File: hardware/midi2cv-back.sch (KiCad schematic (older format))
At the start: 3 parts

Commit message: Add amplifier circuits for DACs
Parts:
- removed U?: STM32F103C8Tx, Package_QFP:LQFP-48_7x7mm_P0.5mm, symbol MCU_ST_STM32F1:STM32F103C8Tx
- added U?: STM32F410RBTx, Package_QFP:LQFP-64_10x10mm_P0.5mm, symbol MCU_ST_STM32F4:STM32F410RBTx
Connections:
- wire segments 29 -> 33
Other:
- moved on the sheet: C?, U?
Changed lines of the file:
@@
 L power:GND #PWR?
 U 1 1 60A4D09B
-P 4250 4750
-F 0 "#PWR?" H 4250 4500 50  0001 C CNN
-F 1 "GND" H 4255 4577 50  0000 C CNN
-F 2 "" H 4250 4750 50  0001 C CNN
-F 3 "" H 4250 4750 50  0001 C CNN
-	1    4250 4750
+P 2350 4850
+F 0 "#PWR?" H 2350 4600 50  0001 C CNN
+F 1 "GND" H 2355 4677 50  0000 C CNN
+F 2 "" H 2350 4850 50  0001 C CNN
+F 3 "" H 2350 4850 50  0001 C CNN
+	1    2350 4850
 	1    0    0    -1
 $EndComp
 Wire Wire Line
-	3850 4100 3850 4200
+	1950 4200 1950 4300
 Wire Wire Line
-	3850 4600 4250 4600
+	1950 4700 2350 4700
 Wire Wire Line
-	4250 4600 4250 4500
-Connection ~ 3850 4200
+	2350 4700 2350 4600
+Connection ~ 1950 4300
 Wire Wire Line
-	3850 4200 3850 4300
-Connection ~ 3850 4300
+	1950 4300 1950 4400
+Connection ~ 1950 4400
 Wire Wire Line
-	3850 4300 3850 4600
+	1950 4400 1950 4700
 Wire Wire Line
-	4250 4600 4250 4750
-Connection ~ 4250 4600
+	2350 4700 2350 4850
+Connection ~ 2350 4700
 Wire Wire Line
-	4250 4600 4650 4600
+	2350 4700 2750 4700
 Wire Wire Line
-	4650 4600 4650 4300
+	2750 4700 2750 4400
 $Comp
 L power:+3.3V #PWR?
 U 1 1 60A52E41
-P 4250 3900
-F 0 "#PWR?" H 4250 3750 50  0001 C CNN
-F 1 "+3.3V" H 4265 4073 50  0000 C CNN
-F 2 "" H 4250 3900 50  0001 C CNN
-F 3 "" H 4250 3900 50  0001 C CNN
-	1    4250 3900
+P 2350 4000
+F 0 "#PWR?" H 2350 3850 50  0001 C CNN
+F 1 "+3.3V" H 2365 4173 50  0000 C CNN
+F 2 "" H 2350 4000 50  0001 C CNN
+F 3 "" H 2350 4000 50  0001 C CNN
+	1    2350 4000
 	1    0    0    -1
 $EndComp
 Wire Wire Line
-	4650 4100 5300 4100
+	2750 4200 3400 4200
 Wire Wire Line
-	4650 4200 5300 4200
+	2750 4300 3400 4300
 $Comp
 L power:+3.3V #PWR?
 U 1 1 60A58EE0
-P 3350 3950
-F 0 "#PWR?" H 3350 3800 50  0001 C CNN
-F 1 "+3.3V" H 3365 4123 50  0000 C CNN
-F 2 "" H 3350 3950 50  0001 C CNN
-F 3 "" H 3350 3950 50  0001 C CNN
-	1    3350 3950
+P 1450 4050
+F 0 "#PWR?" H 1450 3900 50  0001 C CNN
+F 1 "+3.3V" H 1465 4223 50  0000 C CNN
+F 2 "" H 1450 4050 50  0001 C CNN
+F 3 "" H 1450 4050 50  0001 C CNN
+	1    1450 4050
 	1    0    0    -1
 $EndComp
@@
 L power:GND #PWR?
 U 1 1 60A592F0
-P 3350 4250
-F 0 "#PWR?" H 3350 4000 50  0001 C CNN
-F 1 "GND" H 3355 4077 50  0000 C CNN
-F 2 "" H 3350 4250 50  0001 C CNN
-F 3 "" H 3350 4250 50  0001 C CNN
-	1    3350 4250
+P 1450 4350
+F 0 "#PWR?" H 1450 4100 50  0001 C CNN
+F 1 "GND" H 1455 4177 50  0000 C CNN
+F 2 "" H 1450 4350 50  0001 C CNN
+F 3 "" H 1450 4350 50  0001 C CNN
+	1    1450 4350
 	1    0    0    -1
 $EndComp
@@
 L Device:C C?
 U 1 1 60A598C4
-P 3350 4100
-F 0 "C?" H 3465 4146 50  0000 L CNN
-F 1 "100n" H 3465 4055 50  0000 L CNN
-F 2 "" H 3388 3950 50  0001 C CNN
-F 3 "~" H 3350 4100 50  0001 C CNN
-	1    3350 4100
+P 1450 4200
+F 0 "C?" H 1565 4246 50  0000 L CNN
+F 1 "100n" H 1565 4155 50  0000 L CNN
+F 2 "" H 1488 4050 50  0001 C CNN
+F 3 "~" H 1450 4200 50  0001 C CNN
+	1    1450 4200
 	1    0    0    -1
 $EndComp
@@
 L power:+3.3V #PWR?
 U 1 1 60A5CF6A
-P 6000 1800
-F 0 "#PWR?" H 6000 1650 50  0001 C CNN
-F 1 "+3.3V" H 6015 1973 50  0000 C CNN
-F 2 "" H 6000 1800 50  0001 C CNN
-F 3 "" H 6000 1800 50  0001 C CNN
-	1    6000 1800
+P 5600 1400
+F 0 "#PWR?" H 5600 1250 50  0001 C CNN
+F 1 "+3.3V" H 5615 1573 50  0000 C CNN
+F 2 "" H 5600 1400 50  0001 C CNN
+F 3 "" H 5600 1400 50  0001 C CNN
+	1    5600 1400
 	1    0    0    -1
 $EndComp
 Wire Wire Line
-	6000 1800 6000 1900
+	5350 1700 5350 1500
 Wire Wire Line
-	5800 2100 5800 1900
+	5350 1500 5450 1500
+Connection ~ 5550 1500
 Wire Wire Line
-	5800 1900 5900 1900
-Connection ~ 6000 1900
+	5550 1500 5550 1700
 Wire Wire Line
-	6000 1900 6000 2100
+	5450 1700 5450 1500
+Connection ~ 5450 1500
 Wire Wire Line
-	5900 2100 5900 1900
-Connection ~ 5900 1900
+	5450 1500 5550 1500
 Wire Wire Line
-	5900 1900 6000 1900
+	5650 1700 5650 1500
 Wire Wire Line
-	6100 2100 6100 1900
+	5650 1500 5600 1500
 Wire Wire Line
-	6100 1900 6000 1900
+	5750 1700 5750 1500
 Wire Wire Line
-	6200 2100 6200 1900
+	5750 1500 5650 1500
+Connection ~ 5650 1500
 Wire Wire Line
-	6200 1900 6100 1900
-Connection ~ 6100 1900
-Wire Wire Line
-	5900 5100 5900 5300
+	5450 5300 5450 5500
 $Comp
 L Memory_EEPROM:CAT24C256 U?
 U 1 1 60A44E16
-P 4250 4200
-F 0 "U?" H 3850 4600 50  0000 C CNN
-F 1 "AT24C256C" H 3850 4500 50  0000 C CNN
-F 2 "" H 4250 4200 50  0001 C CNN
-F 3 "https://www.onsemi.cn/PowerSolutions/document/CAT24C256-D.PDF" H 4250 4200 50  0001 C CNN
-	1    4250 4200
+P 2350 4300
+F 0 "U?" H 1950 4700 50  0000 C CNN
+F 1 "AT24C256C" H 1950 4600 50  0000 C CNN
+F 2 "" H 2350 4300 50  0001 C CNN
+F 3 "https://www.onsemi.cn/PowerSolutions/document/CAT24C256-D.PDF" H 2350 4300 50  0001 C CNN
+	1    2350 4300
 	1    0    0    -1
 $EndComp
 Wire Wire Line
-	5800 5100 5800 5300
+	5350 5300 5350 5500
 Wire Wire Line
-	5800 5300 5900 5300
+	5350 5500 5450 5500
 Wire Wire Line
-	6000 5300 6000 5100
-Connection ~ 5900 5300
+	5550 5500 5550 5300
+Connection ~ 5450 5500
 Wire Wire Line
-	6000 5300 6100 5300
+	5550 5500 5650 5500
 Wire Wire Line
-	6100 5300 6100 5100
-Connection ~ 6000 5300
-$Comp
-L MCU_ST_STM32F1:STM32F103C8Tx U?
-U 1 1 60A44151
-P 6000 3600
-F 0 "U?" H 6550 2050 50  0000 C CNN
-F 1 "STM32F103C8Tx" H 6550 1950 50  0000 C CNN
-F 2 "Package_QFP:LQFP-48_7x7mm_P0.5mm" H 5400 2200 50  0001 R CNN
-F 3 "http://www.st.com/st-web-ui/static/active/en/resource/technical/document/datasheet/CD00161566.pdf" H 6000 3600 50  0001 C CNN
-	1    6000 3600
-	1    0    0    -1
-$EndComp
+	5650 5500 5650 5300
+Connection ~ 5550 5500
 $Comp
 L power:GND #PWR?
 U 1 1 60A664FC
-P 5950 5400
-F 0 "#PWR?" H 5950 5150 50  0001 C CNN
-F 1 "GND" H 5955 5227 50  0000 C CNN
-F 2 "" H 5950 5400 50  0001 C CNN
-F 3 "" H 5950 5400 50  0001 C CNN
-	1    5950 5400
+P 5550 5600
+F 0 "#PWR?" H 5550 5350 50  0001 C CNN
+F 1 "GND" H 5555 5427 50  0000 C CNN
+F 2 "" H 5550 5600 50  0001 C CNN
+F 3 "" H 5550 5600 50  0001 C CNN
+	1    5550 5600
 	1    0    0    -1
 $EndComp
-Wire Wire Line
-	5900 5300 5950 5300
-Wire Wire Line
-	5950 5300 5950 5400
-Connection ~ 5950 5300
-Wire Wire Line
-	5950 5300 6000 5300
-Text GLabel 6600 3900 2    50   Input ~ 0
+Text GLabel 3500 5700 2    50   Input ~ 0
 spi1_sck
 Text GLabel 8500 2600 0    50   Input ~ 0
 spi1_sck
-Text GLabel 6600 3800 2    50   Input ~ 0
+Text GLabel 3500 5600 2    50   Input ~ 0
 spi1_nss
 Text GLabel 8500 2750 0    50   Input ~ 0
 spi1_nss
-Text GLabel 6600 4100 2    50   Input ~ 0
+Text GLabel 3500 5900 2    50   Input ~ 0
 spi1_mosi
 Text GLabel 8500 2450 0    50   Input ~ 0
 spi1_mosi
-Text GLabel 5300 4400 0    50   Input ~ 0
+Text GLabel 3900 5050 0    50   Input ~ 0
 i2c2_scl
-Text GLabel 5300 4500 0    50   Input ~ 0
+Text GLabel 3900 5150 0    50   Input ~ 0
 i2c2_sda
 Text GLabel 8500 4250 0    50   Input ~ 0
@@
 Text GLabel 8500 4450 0    50   Input ~ 0
 i2c2_sda
+$Comp
+L MCU_ST_STM32F4:STM32F410RBTx U?
+U 1 1 60B028B6
+P 5550 3500
+F 0 "U?" H 6150 1650 50  0000 C CNN
+F 1 "STM32F410RBTx" H 6150 1550 50  0000 C CNN
+F 2 "Package_QFP:LQFP-64_10x10mm_P0.5mm" H 4950 1800 50  0001 R CNN
+F 3 "http://www.st.com/st-web-ui/static/active/en/resource/technical/document/datasheet/DM00214043.pdf" H 5550 3500 50  0001 C CNN
+	1    5550 3500
+	1    0    0    -1
+$EndComp
+Wire Wire Line
+	5750 1500 5850 1500
+Wire Wire Line
+	5850 1500 5850 1700
+Connection ~ 5750 1500
+Wire Wire Line
+	5600 1500 5600 1400
+Connection ~ 5600 1500
+Wire Wire Line
+	5600 1500 5550 1500
+Wire Wire Line
+	5650 5500 5750 5500
+Wire Wire Line
+	5750 5500 5750 5300
+Connection ~ 5650 5500
+Wire Wire Line
+	5450 5500 5550 5500
+Wire Wire Line
+	5550 5500 5550 5600
 $EndSCHEMATC

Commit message: Move to single schema tree
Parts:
- removed U?: STM32F410RBTx, Package_QFP:LQFP-64_10x10mm_P0.5mm, symbol MCU_ST_STM32F4:STM32F410RBTx
- added U?: STM32F401RBTx, Package_QFP:LQFP-64_10x10mm_P0.5mm, symbol MCU_ST_STM32F4:STM32F401RBTx
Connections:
- wire segments 33 -> 30
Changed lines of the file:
@@
 $Descr A4 11693 8268
 encoding utf-8
-Sheet 1 3
+Sheet 2 5
 Title ""
 Date ""
@@
 L power:+3.3V #PWR?
 U 1 1 60A5CF6A
-P 5600 1400
-F 0 "#PWR?" H 5600 1250 50  0001 C CNN
-F 1 "+3.3V" H 5615 1573 50  0000 C CNN
-F 2 "" H 5600 1400 50  0001 C CNN
-F 3 "" H 5600 1400 50  0001 C CNN
-	1    5600 1400
-	1    0    0    -1
-$EndComp
-Wire Wire Line
-	5350 1700 5350 1500
-Wire Wire Line
-	5350 1500 5450 1500
-Connection ~ 5550 1500
-Wire Wire Line
-	5550 1500 5550 1700
-Wire Wire Line
-	5450 1700 5450 1500
-Connection ~ 5450 1500
-Wire Wire Line
-	5450 1500 5550 1500
-Wire Wire Line
-	5650 1700 5650 1500
-Wire Wire Line
-	5650 1500 5600 1500
-Wire Wire Line
-	5750 1700 5750 1500
-Wire Wire Line
-	5750 1500 5650 1500
-Connection ~ 5650 1500
+P 5550 1600
+F 0 "#PWR?" H 5550 1450 50  0001 C CNN
+F 1 "+3.3V" H 5565 1773 50  0000 C CNN
+F 2 "" H 5550 1600 50  0001 C CNN
+F 3 "" H 5550 1600 50  0001 C CNN
+	1    5550 1600
+	1    0    0    -1
+$EndComp
 Wire Wire Line
 	5450 5300 5450 5500
@@
 	1    0    0    -1
 $EndComp
-Text GLabel 3500 5700 2    50   Input ~ 0
+Text GLabel 3700 3650 2    50   Input ~ 0
 spi1_sck
 Text GLabel 8500 2600 0    50   Input ~ 0
 spi1_sck
-Text GLabel 3500 5600 2    50   Input ~ 0
+Text GLabel 3700 3550 2    50   Input ~ 0
 spi1_nss
 Text GLabel 8500 2750 0    50   Input ~ 0
 spi1_nss
-Text GLabel 3500 5900 2    50   Input ~ 0
+Text GLabel 3700 3850 2    50   Input ~ 0
 spi1_mosi
 Text GLabel 8500 2450 0    50   Input ~ 0
 spi1_mosi
-Text GLabel 3900 5050 0    50   Input ~ 0
+Text GLabel 4100 3000 0    50   Input ~ 0
 i2c2_scl
-Text GLabel 3900 5150 0    50   Input ~ 0
+Text GLabel 4100 3100 0    50   Input ~ 0
 i2c2_sda
 Text GLabel 8500 4250 0    50   Input ~ 0
@@
 Text GLabel 8500 4450 0    50   Input ~ 0
 i2c2_sda
-$Comp
-L MCU_ST_STM32F4:STM32F410RBTx U?
-U 1 1 60B028B6
-P 5550 3500
-F 0 "U?" H 6150 1650 50  0000 C CNN
-F 1 "STM32F410RBTx" H 6150 1550 50  0000 C CNN
-F 2 "Package_QFP:LQFP-64_10x10mm_P0.5mm" H 4950 1800 50  0001 R CNN
-F 3 "http://www.st.com/st-web-ui/static/active/en/resource/technical/document/datasheet/DM00214043.pdf" H 5550 3500 50  0001 C CNN
-	1    5550 3500
-	1    0    0    -1
-$EndComp
-Wire Wire Line
-	5750 1500 5850 1500
-Wire Wire Line
-	5850 1500 5850 1700
-Connection ~ 5750 1500
-Wire Wire Line
-	5600 1500 5600 1400
-Connection ~ 5600 1500
-Wire Wire Line
-	5600 1500 5550 1500
 Wire Wire Line
 	5650 5500 5750 5500
@@
 Wire Wire Line
 	5550 5500 5550 5600
+$Comp
+L MCU_ST_STM32F4:STM32F401RBTx U?
+U 1 1 6100D1FD
+P 5550 3500
+F 0 "U?" H 6250 5300 50  0000 C CNN
+F 1 "STM32F401RBTx" H 6250 5200 50  0000 C CNN
+F 2 "Package_QFP:LQFP-64_10x10mm_P0.5mm" H 4950 1800 50  0001 R CNN
+F 3 "http://www.st.com/st-web-ui/static/active/en/resource/technical/document/datasheet/DM00086815.pdf" H 5550 3500 50  0001 C CNN
+	1    5550 3500
+	1    0    0    -1
+$EndComp
+Wire Wire Line
+	5550 1600 5550 1700
+Wire Wire Line
+	5550 1700 5650 1700
+Wire Wire Line
+	5650 1700 5650 1800
+Connection ~ 5550 1700
+Wire Wire Line
+	5550 1700 5550 1800
+Wire Wire Line
+	5650 1700 5750 1700
+Wire Wire Line
+	5750 1700 5750 1800
+Connection ~ 5650 1700
+Wire Wire Line
+	5550 1700 5450 1700
+Wire Wire Line
+	5450 1700 5450 1800
+Wire Wire Line
+	5450 1700 5350 1700
+Wire Wire Line
+	5350 1700 5350 1800
+Connection ~ 5450 1700
 $EndSCHEMATC

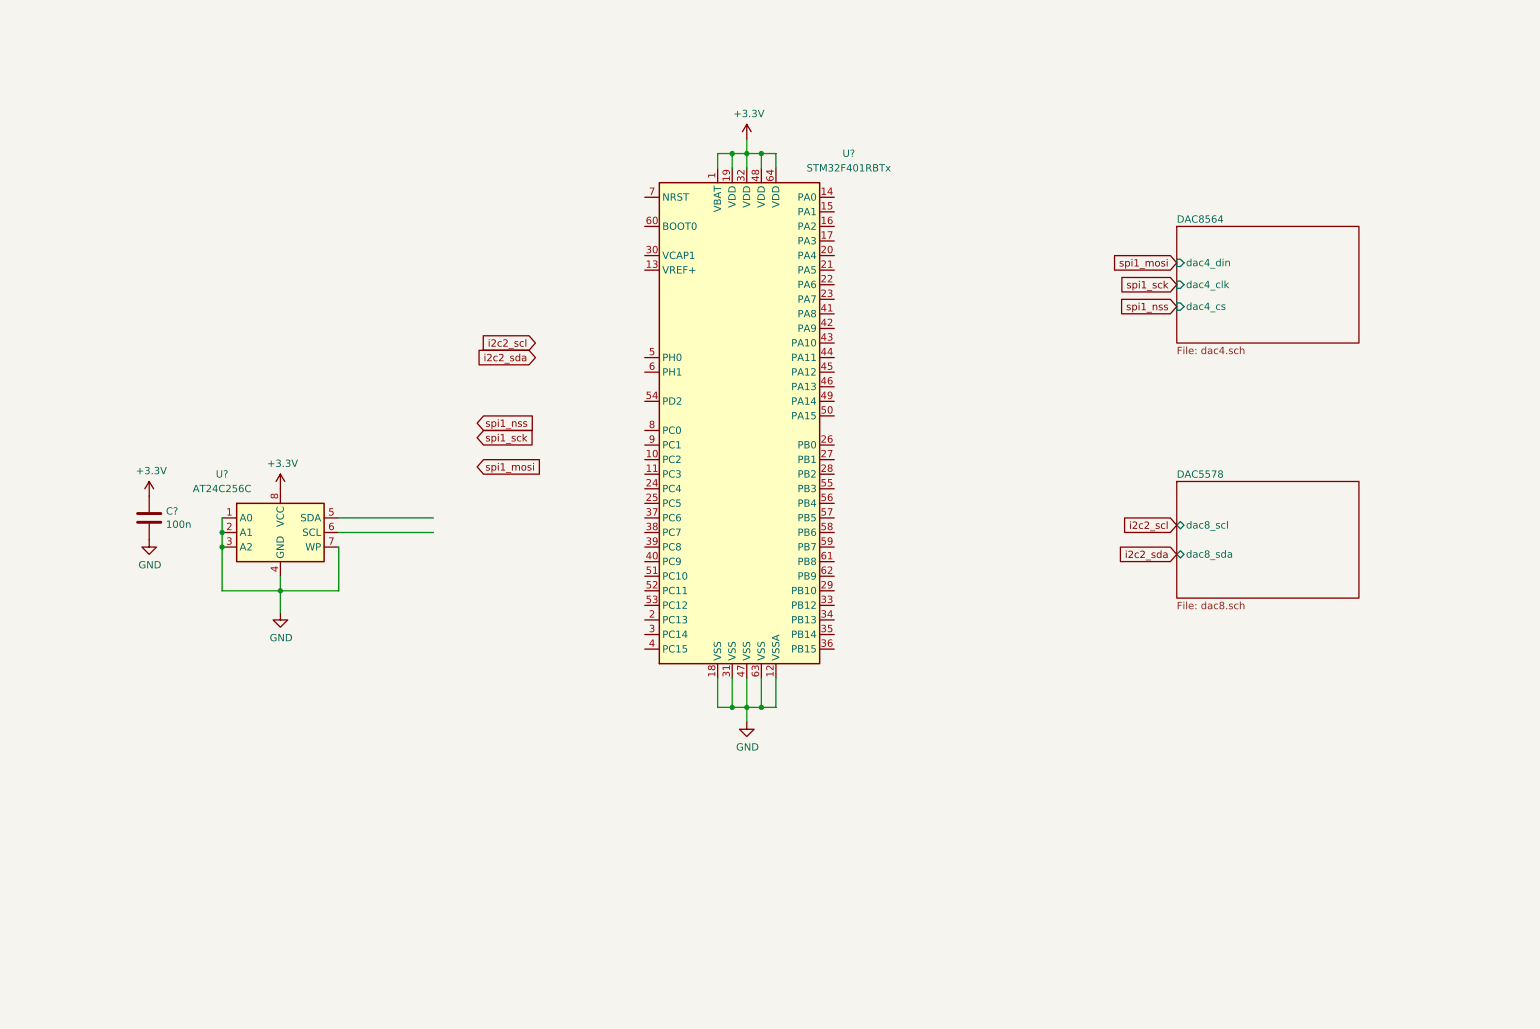
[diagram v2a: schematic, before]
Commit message: First preliminary board design
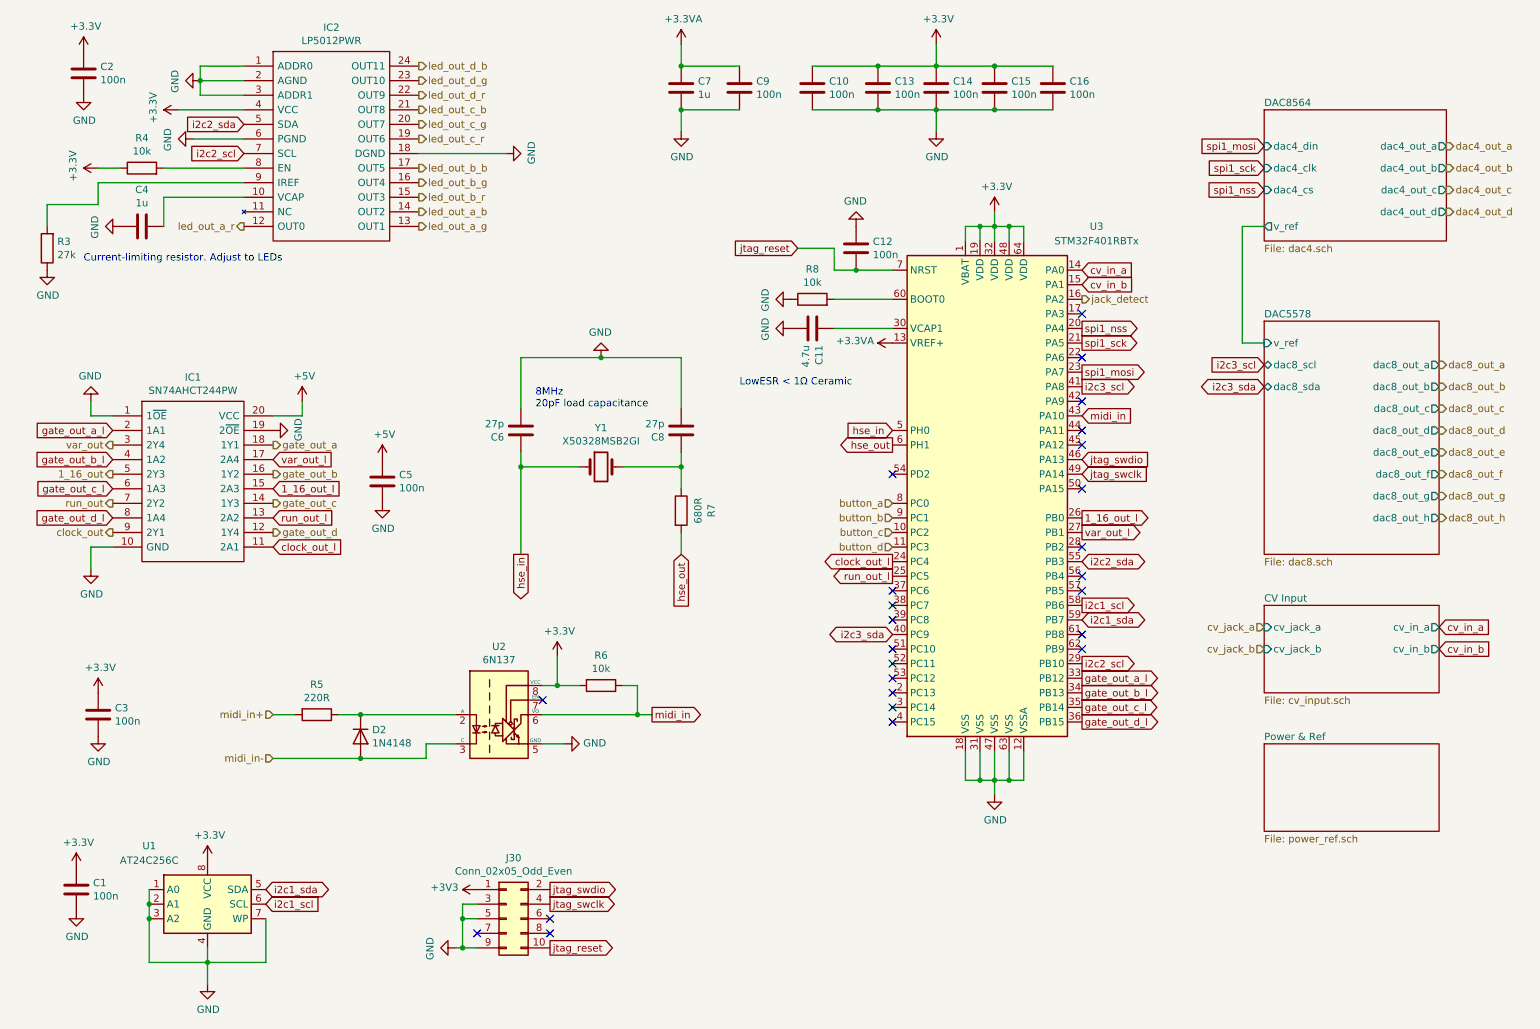
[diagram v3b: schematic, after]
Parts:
- added C10, C12, C13, C14, C15, C16, C2, C3, C5, C9: 100n, Capacitor_SMD:C_0603_1608Metric, symbol Device:C
- added C11: 4.7u, Capacitor_SMD:C_0603_1608Metric, symbol Device:C
- added C4, C7: 1u, Capacitor_SMD:C_0603_1608Metric, symbol Device:C
- added C6, C8: 27p, Capacitor_SMD:C_0603_1608Metric, symbol Device:C
- added D2: 1N4148, Diode_SMD:D_SOD-123, symbol Diode:1N4148
- added IC1: SN74AHCT244PW, SN74AHCT244PW:SOP65P640X120-20N, symbol SN74AHCT244PW:SN74AHCT244PW
- added IC2: LP5012PWR, LP5012PWR:SOP65P640X120-24N, symbol LP5012PWR:LP5012PWR
- added J30: Conn_02x05_Odd_Even, Connector_PinHeader_1.27mm:PinHeader_2x05_P1.27mm_Vertical, symbol Connector_Generic:Conn_02x05_Odd_Even
- added R3: 27k, Resistor_SMD:R_0603_1608Metric_Pad0.98x0.95mm_HandSolder, symbol Device:R
- added R4, R6, R8: 10k, Resistor_SMD:R_0603_1608Metric, symbol Device:R
- added R5: 220R, Resistor_SMD:R_0603_1608Metric, symbol Device:R
- added R7: 680R, Resistor_SMD:R_0603_1608Metric, symbol Device:R
- added U2: 6N137, Package_DIP:SMDIP-8_W9.53mm, symbol Isolator:6N137
- added Y1: X50328MSB2GI, Crystal:Crystal_SMD_5032-2Pin_5.0x3.2mm, symbol Device:Crystal
- C1: renamed from C?; footprint (none) -> Capacitor_SMD:C_0603_1608Metric
- U1: renamed from U?; footprint (none) -> Package_SO:SOIC-8_3.9x4.9mm_P1.27mm
- gave numbers to parts that had none: 1
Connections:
- net labels added: +3.3VA, +3V3, +5V, 1_16_out, 1_16_out_l, button_a, button_b, button_c, button_d, clock_out, clock_out_l, cv_in_a, cv_in_b, cv_jack_a, cv_jack_b, dac4_out_a, dac4_out_b, dac4_out_c, dac4_out_d, dac8_out_a, dac8_out_b, dac8_out_c, dac8_out_d, dac8_out_e, dac8_out_f, dac8_out_g, dac8_out_h, gate_out_a, gate_out_a_l, gate_out_b, gate_out_b_l, gate_out_c, gate_out_c_l, gate_out_d, gate_out_d_l, hse_in, hse_out, i2c1_scl, i2c1_sda, i2c3_scl, i2c3_sda, jack_detect, jtag_reset, jtag_swclk, jtag_swdio, led_out_a_b, led_out_a_g, led_out_a_r, led_out_b_b, led_out_b_g, led_out_b_r, led_out_c_b, led_out_c_g, led_out_c_r, led_out_d_b, led_out_d_g, led_out_d_r, midi_in, midi_in+, midi_in-, run_out, run_out_l, var_out, var_out_l
- wire segments 30 -> 105
- no-connect marks 0 -> 25
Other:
- note added: "8MHz\n20pF load capacitance"
- note added: "Current-limiting resistor. Adjust to LEDs"
- note added: "LowESR < 1Ω Ceramic"
- moved on the sheet: C1, U1, U3
